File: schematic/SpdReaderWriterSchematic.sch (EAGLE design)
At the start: 16 parts, among them IC1 9V Boost Converter, U1 EEPROM

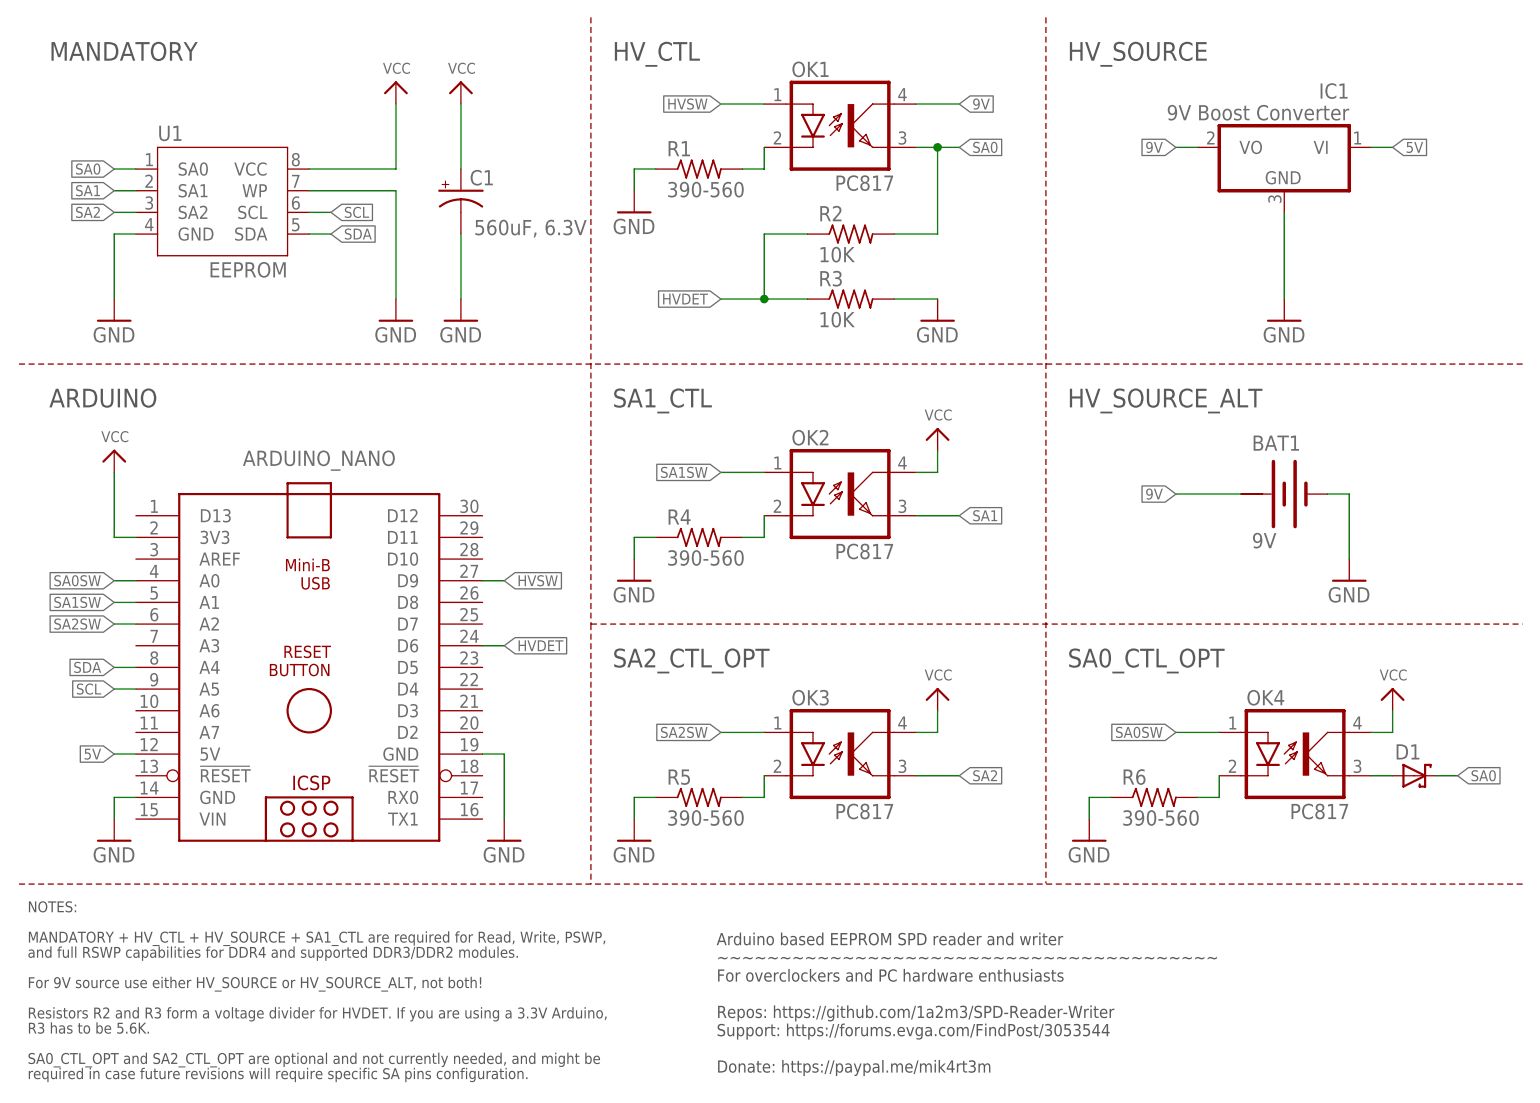
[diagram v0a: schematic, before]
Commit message: Add files via upload
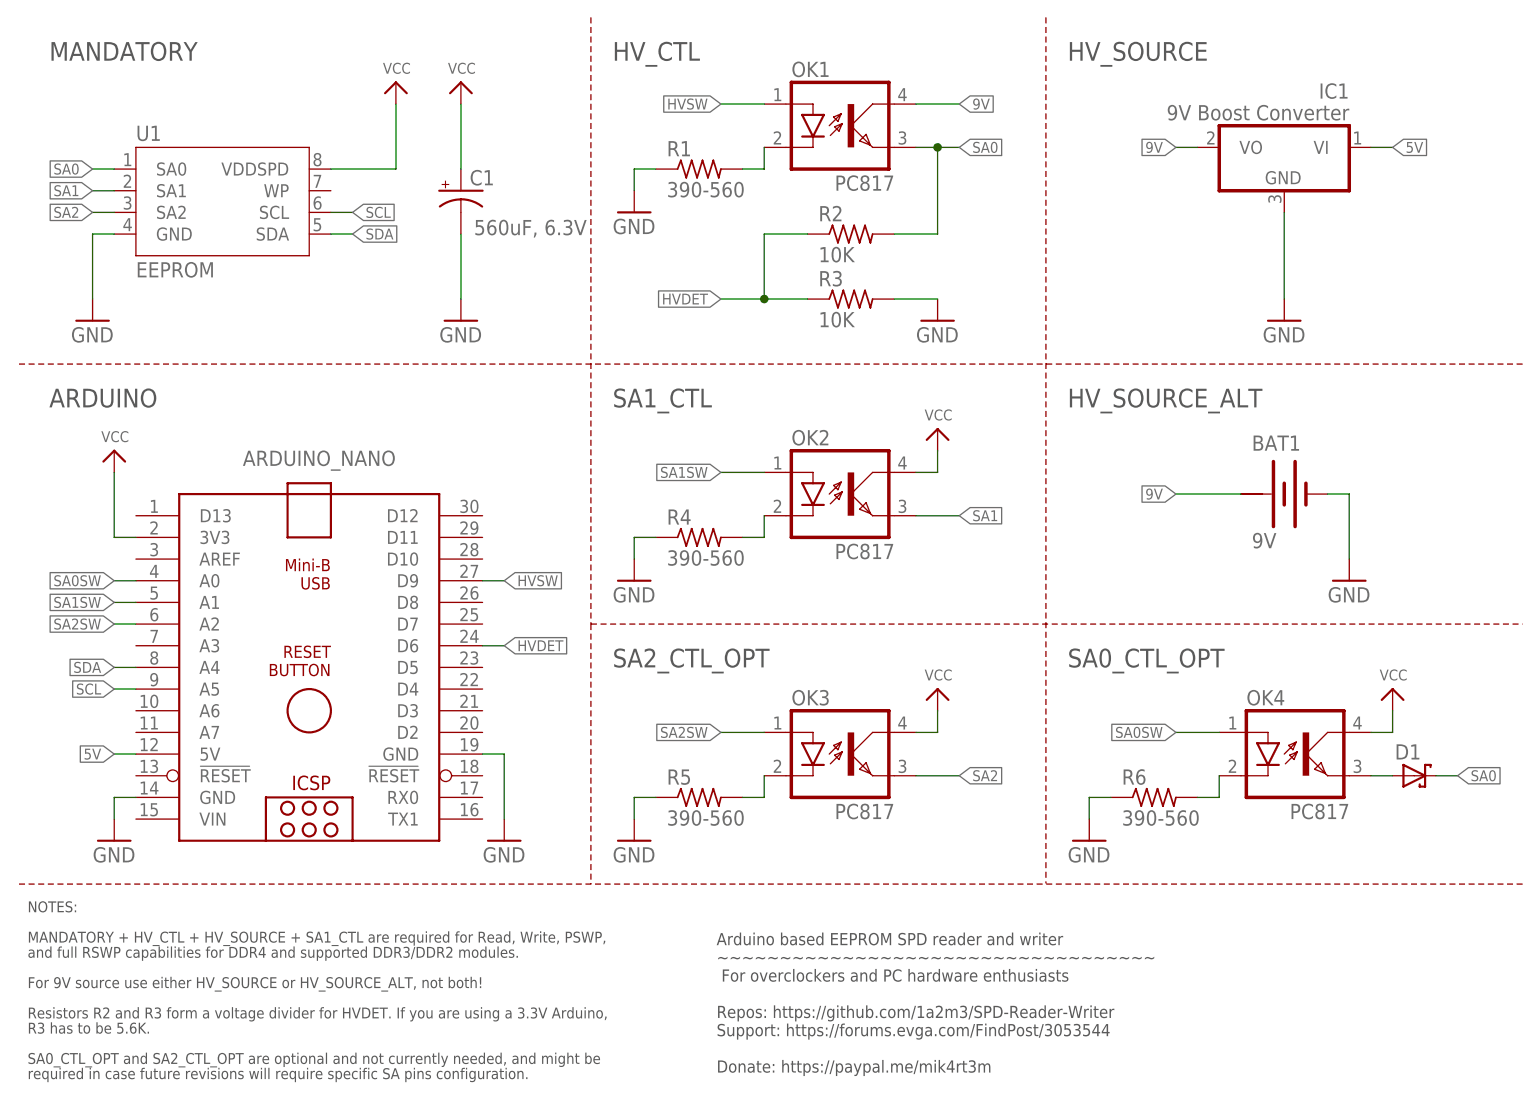
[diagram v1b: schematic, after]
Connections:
- net GND: no longer U1.WP
- net VCC: now also U1.VDDSPD; no longer U1.VCC
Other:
- note added: "Arduino based EEPROM SPD reader and writer ~~~~~~~~~~~~~~~~~~~~~~~~~~~~~~~~~~~ For overclockers and PC hardware enthusiasts Repos: https://github.com/1a2m3/SPD-Reader-Writer Support: https://forums.evga.com/FindPost/3053544 Donate: https://paypal.me/mik4rt3m"
- note removed: "Arduino based EEPROM SPD reader and writer ~~~~~~~~~~~~~~~~~~~~~~~~~~~~~~~~~~~~~~~~ For overclockers and PC hardware enthusiasts Repos: https://github.com/1a2m3/SPD-Reader-Writer Support: https://forums.evga.com/FindPost/3053544 Donate: https://paypal.me/mik4rt3m"
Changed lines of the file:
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@@
 <part name="BAT1" library="special" library_urn="urn:adsk.eagle:library:367" deviceset="BATTERY" device="" package3d_urn="urn:adsk.eagle:package:26670/1" value="9V"/>
 <part name="P+5" library="audio amplifier example" library_urn="urn:adsk.eagle:library:970892" deviceset="VCC" device=""/>
-<part name="GND12" library="supply1" library_urn="urn:adsk.eagle:library:371" deviceset="GND" device=""/>
-<part name="U1" library="EEPROM" deviceset="EEPROM" device=""/>
 <part name="GND14" library="supply1" library_urn="urn:adsk.eagle:library:371" deviceset="GND" device=""/>
 <part name="R2" library="adafruit" library_urn="urn:adsk.eagle:library:420" deviceset="R-US_" device="0204/7" package3d_urn="urn:adsk.eagle:package:6240596/1" value="10K"/>
@@
 <part name="GND10" library="supply1" library_urn="urn:adsk.eagle:library:371" deviceset="GND" device=""/>
 <part name="D1" library="adafruit" library_urn="urn:adsk.eagle:library:420" deviceset="SCHOTTKY-DIODE" device="DO35-7" package3d_urn="urn:adsk.eagle:package:6240681/1"/>
+<part name="U1" library="EEPROM" deviceset="EEPROM" device=""/>
 </parts>
 <sheets>
@@
 <text x="7.62" y="83.82" size="2.1844" layer="97" font="vector">ARDUINO</text>
 <wire x1="180.34" y1="27.94" x2="3.8862" y2="27.94" width="0.0762" layer="94" style="shortdash"/>
-<text x="85.852" y="5.842" size="1.4224" layer="97" font="vector">Arduino based EEPROM SPD reader and writer
-~~~~~~~~~~~~~~~~~~~~~~~~~~~~~~~~~~~~~~~~
-For overclockers and PC hardware enthusiasts
+<text x="85.852" y="5.842" size="1.4224" layer="97">Arduino based EEPROM SPD reader and writer
+~~~~~~~~~~~~~~~~~~~~~~~~~~~~~~~~~~~
+ For overclockers and PC hardware enthusiasts
 Repos: https://github.com/1a2m3/SPD-Reader-Writer
 Support: https://forums.evga.com/FindPost/3053544
@@
 <attribute name="VALUE" x="58.42" y="30.48" size="1.778" layer="96"/>
 </instance>
-<instance part="GND7" gate="1" x="15.24" y="93.98" smashed="yes">
-<attribute name="VALUE" x="12.7" y="91.44" size="1.778" layer="96"/>
+<instance part="GND7" gate="1" x="12.7" y="93.98" smashed="yes">
+<attribute name="VALUE" x="10.16" y="91.44" size="1.778" layer="96"/>
 </instance>
 <instance part="OK2" gate="G$1" x="101.6" y="73.66" smashed="yes">
@@
 <instance part="P+5" gate="VCC" x="48.26" y="121.92" smashed="yes">
 <attribute name="VALUE" x="46.736" y="122.936" size="1.27" layer="96"/>
-</instance>
-<instance part="GND12" gate="1" x="48.26" y="93.98" smashed="yes">
-<attribute name="VALUE" x="45.72" y="91.44" size="1.778" layer="96"/>
-</instance>
-<instance part="U1" gate="G$1" x="27.94" y="106.68" smashed="yes">
-<attribute name="NAME" x="20.32" y="116.84" size="1.778" layer="95" rot="R180" align="bottom-right"/>
-<attribute name="VALUE" x="35.56" y="99.06" size="1.778" layer="95" rot="MR0"/>
 </instance>
 <instance part="GND14" gate="1" x="111.76" y="93.98" smashed="yes">
@@
 <attribute name="NAME" x="165.354" y="42.545" size="1.778" layer="95"/>
 <attribute name="VALUE" x="165.354" y="37.211" size="1.778" layer="96"/>
+</instance>
+<instance part="U1" gate="G$1" x="27.94" y="106.68" smashed="yes">
+<attribute name="NAME" x="17.78" y="116.84" size="1.778" layer="95" rot="R180" align="bottom-right"/>
+<attribute name="VALUE" x="17.78" y="99.06" size="1.778" layer="95"/>
 </instance>
 </instances>
@@
 </segment>
 <segment>
-<pinref part="U1" gate="G$1" pin="WP"/>
-<wire x1="38.1" y1="109.22" x2="48.26" y2="109.22" width="0.1524" layer="91"/>
-<pinref part="GND12" gate="1" pin="GND"/>
-<wire x1="48.26" y1="109.22" x2="48.26" y2="96.52" width="0.1524" layer="91"/>
-</segment>
-<segment>
+<wire x1="15.24" y1="104.14" x2="12.7" y2="104.14" width="0.1524" layer="91"/>
+<wire x1="12.7" y1="104.14" x2="12.7" y2="96.52" width="0.1524" layer="91"/>
+<pinref part="GND7" gate="1" pin="GND"/>
 <pinref part="U1" gate="G$1" pin="GND"/>
-<wire x1="17.78" y1="104.14" x2="15.24" y2="104.14" width="0.1524" layer="91"/>
-<wire x1="15.24" y1="104.14" x2="15.24" y2="96.52" width="0.1524" layer="91"/>
-<pinref part="GND7" gate="1" pin="GND"/>
 </segment>
 <segment>
@@
 </segment>
 <segment>
-<pinref part="U1" gate="G$1" pin="VCC"/>
-<wire x1="38.1" y1="111.76" x2="48.26" y2="111.76" width="0.1524" layer="91"/>
+<wire x1="40.64" y1="111.76" x2="48.26" y2="111.76" width="0.1524" layer="91"/>
 <pinref part="P+5" gate="VCC" pin="VCC"/>
 <wire x1="48.26" y1="111.76" x2="48.26" y2="119.38" width="0.1524" layer="91"/>
+<pinref part="U1" gate="G$1" pin="VDDSPD"/>
 </segment>
 <segment>
@@
 </segment>
 <segment>
+<wire x1="15.24" y1="111.76" x2="12.7" y2="111.76" width="0.1524" layer="91"/>
+<label x="12.7" y="111.76" size="1.27" layer="95" rot="R180" xref="yes"/>
 <pinref part="U1" gate="G$1" pin="SA0"/>
-<wire x1="17.78" y1="111.76" x2="15.24" y2="111.76" width="0.1524" layer="91"/>
-<label x="15.24" y="111.76" size="1.27" layer="95" rot="R180" xref="yes"/>
 </segment>
 <segment>
@@
 </segment>
 <segment>
+<wire x1="15.24" y1="109.22" x2="12.7" y2="109.22" width="0.1524" layer="91"/>
+<label x="12.7" y="109.22" size="1.27" layer="95" rot="R180" xref="yes"/>
 <pinref part="U1" gate="G$1" pin="SA1"/>
-<wire x1="17.78" y1="109.22" x2="15.24" y2="109.22" width="0.1524" layer="91"/>
-<label x="15.24" y="109.22" size="1.27" layer="95" rot="R180" xref="yes"/>
 </segment>
 </net>
@@
 </segment>
 <segment>
+<wire x1="40.64" y1="104.14" x2="43.18" y2="104.14" width="0.1524" layer="91"/>
+<label x="43.18" y="104.14" size="1.27" layer="95" xref="yes"/>
 <pinref part="U1" gate="G$1" pin="SDA"/>
-<wire x1="38.1" y1="104.14" x2="40.64" y2="104.14" width="0.1524" layer="91"/>
-<label x="40.64" y="104.14" size="1.27" layer="95" xref="yes"/>
 </segment>
 </net>
@@
 </segment>
 <segment>
+<wire x1="40.64" y1="106.68" x2="43.18" y2="106.68" width="0.1524" layer="91"/>
+<label x="43.18" y="106.68" size="1.27" layer="95" xref="yes"/>
 <pinref part="U1" gate="G$1" pin="SCL"/>
-<wire x1="38.1" y1="106.68" x2="40.64" y2="106.68" width="0.1524" layer="91"/>
-<label x="40.64" y="106.68" size="1.27" layer="95" xref="yes"/>
 </segment>
 </net>
@@
 </segment>
 <segment>
+<wire x1="15.24" y1="106.68" x2="12.7" y2="106.68" width="0.1524" layer="91"/>
+<label x="12.7" y="106.68" size="1.27" layer="95" rot="R180" xref="yes"/>
 <pinref part="U1" gate="G$1" pin="SA2"/>
-<wire x1="17.78" y1="106.68" x2="15.24" y2="106.68" width="0.1524" layer="91"/>
-<label x="15.24" y="106.68" size="1.27" layer="95" rot="R180" xref="yes"/>
-</segment>
-</net>
+</segment>
+</net>
